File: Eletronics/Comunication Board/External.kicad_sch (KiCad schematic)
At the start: 7 parts, among them J2 Conn_01x10_Female

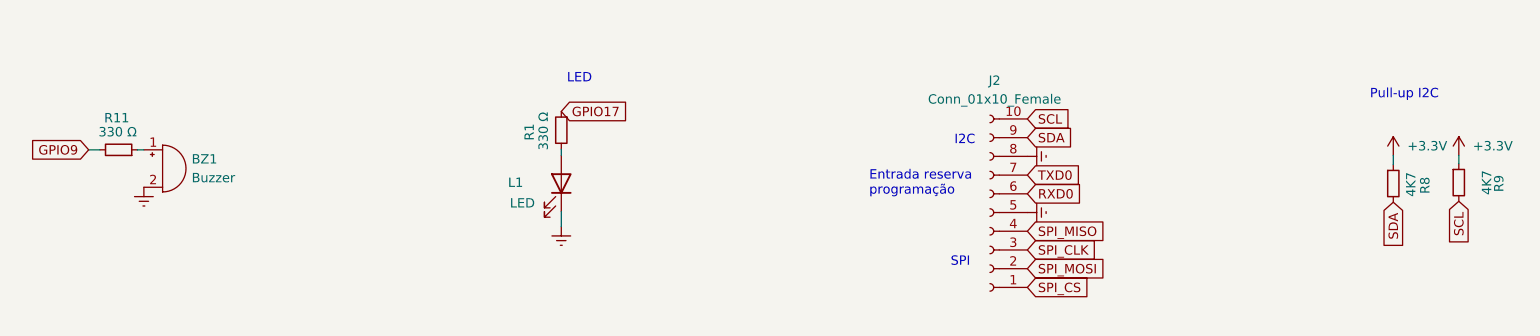
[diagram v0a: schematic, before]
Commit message: alteracoes finais
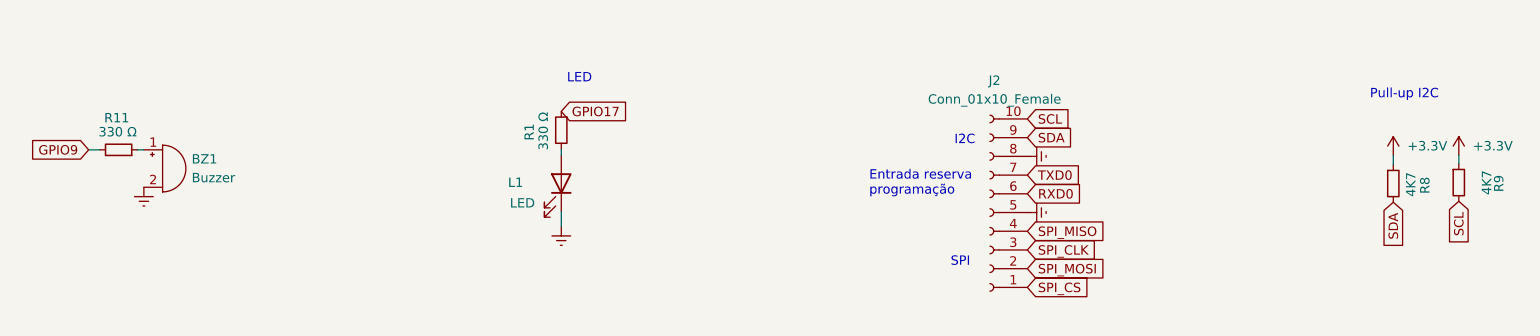
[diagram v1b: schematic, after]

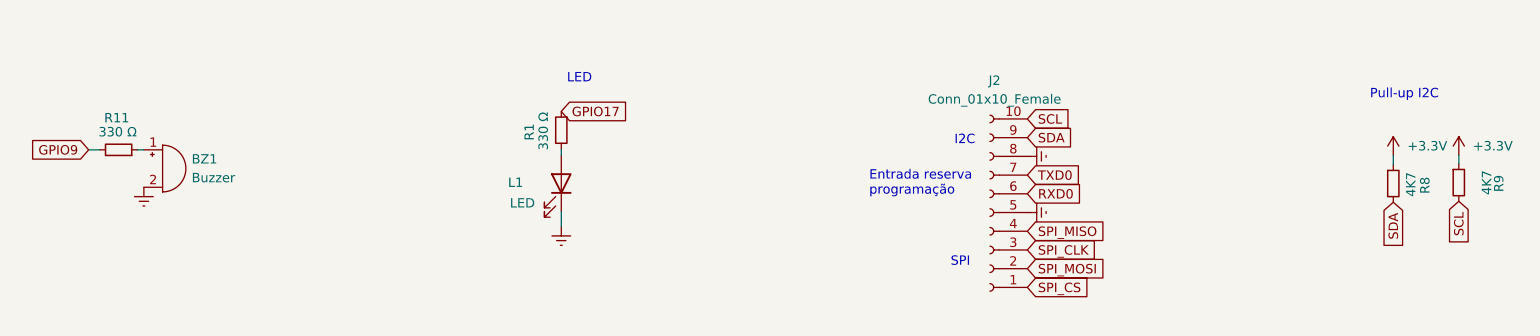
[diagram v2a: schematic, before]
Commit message: edit communication board
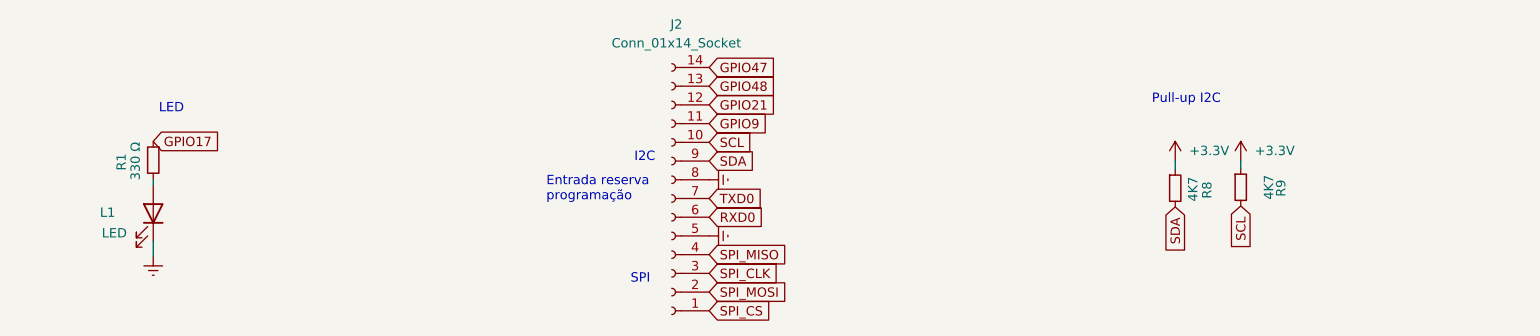
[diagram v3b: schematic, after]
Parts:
- removed BZ1: Buzzer, Buzzer_Beeper:Buzzer_12x9.5RM7.6, symbol Device:Buzzer
- removed J2: Conn_01x10_Female, Connector_IDC:IDC-Header_2x05_P2.54mm_Vertical, symbol Connector:Conn_01x10_Female
- removed R11: 330 Ω, Resistor_SMD:R_0603_1608Metric, symbol Device:R_Small
- added J2: Conn_01x14_Socket, symbol Connector:Conn_01x14_Socket
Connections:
- net GNDREF: now also J2.5 (Pin_5), J2.8 (Pin_8)
- net GPIO9: now also J2.11 (Pin_11)
- net RXD0: now also J2.6 (Pin_6)
- net SCL: now also J2.10 (Pin_10)
- net SDA: now also J2.9 (Pin_9)
- net SPI_CLK: now also J2.3 (Pin_3)
- net SPI_CS: now also J2.1 (Pin_1)
- net SPI_MISO: now also J2.4 (Pin_4)
- net SPI_MOSI: now also J2.2 (Pin_2)
- net TXD0: now also J2.7 (Pin_7)
- new net GPIO21: J2.12 (Pin_12)
- new net GPIO47: J2.14 (Pin_14)
- new net GPIO48: J2.13 (Pin_13)
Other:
- moved on the sheet: L1, R1, R8, R9
